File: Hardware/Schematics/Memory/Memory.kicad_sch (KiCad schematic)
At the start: 5 parts

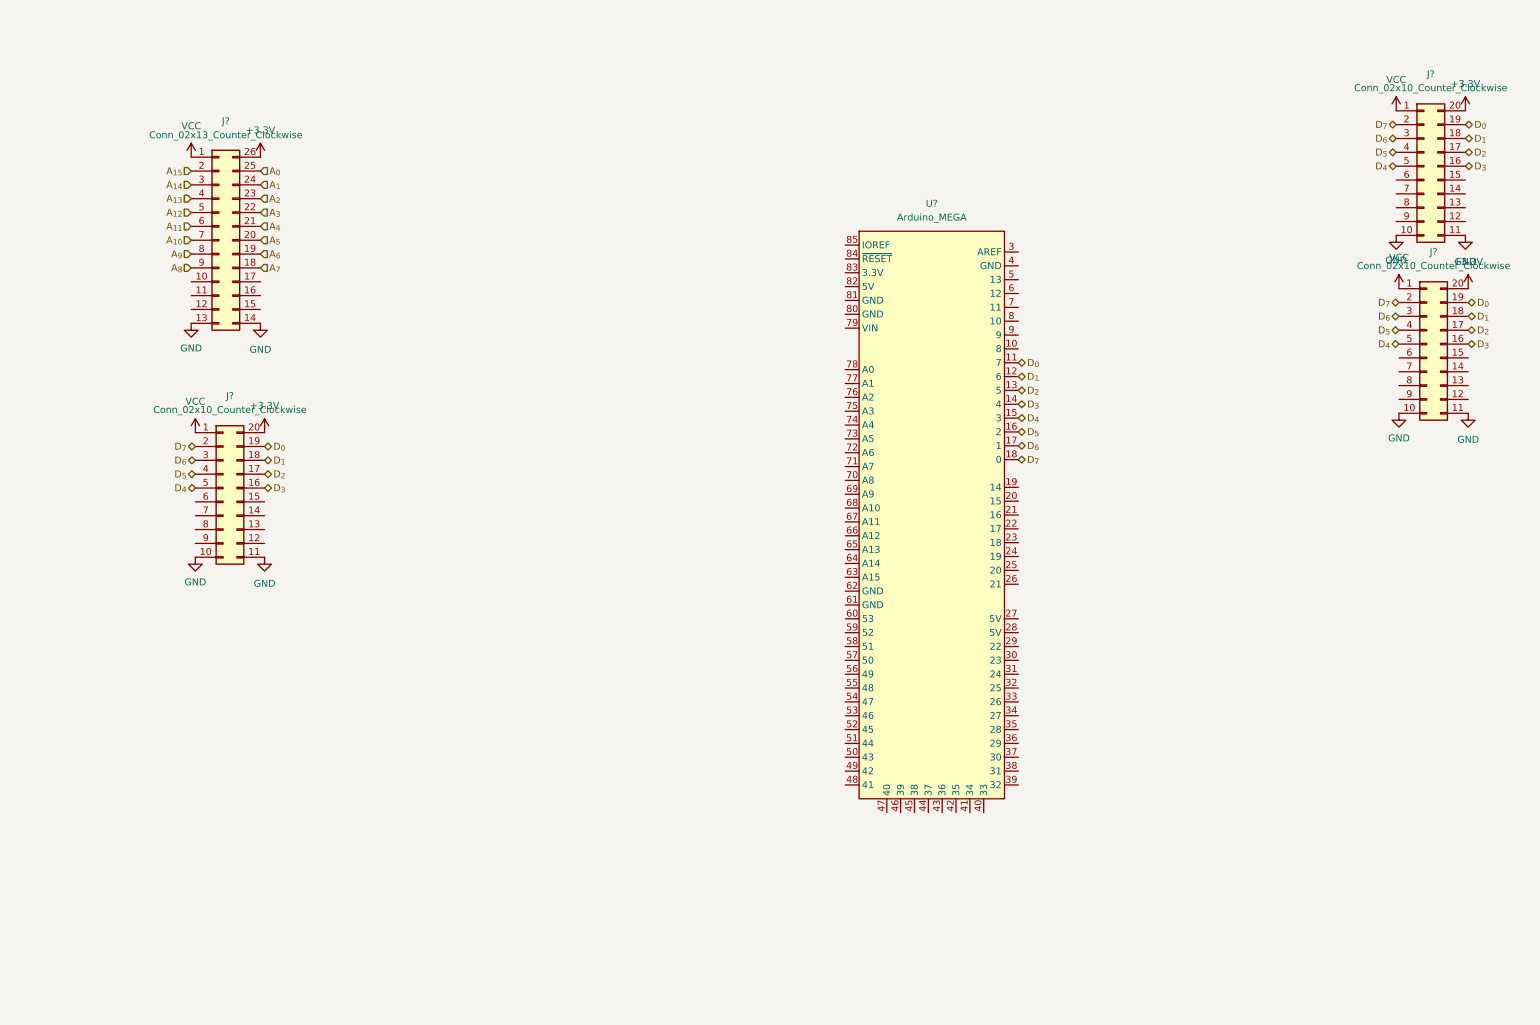
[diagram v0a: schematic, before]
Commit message: Updated Schematics
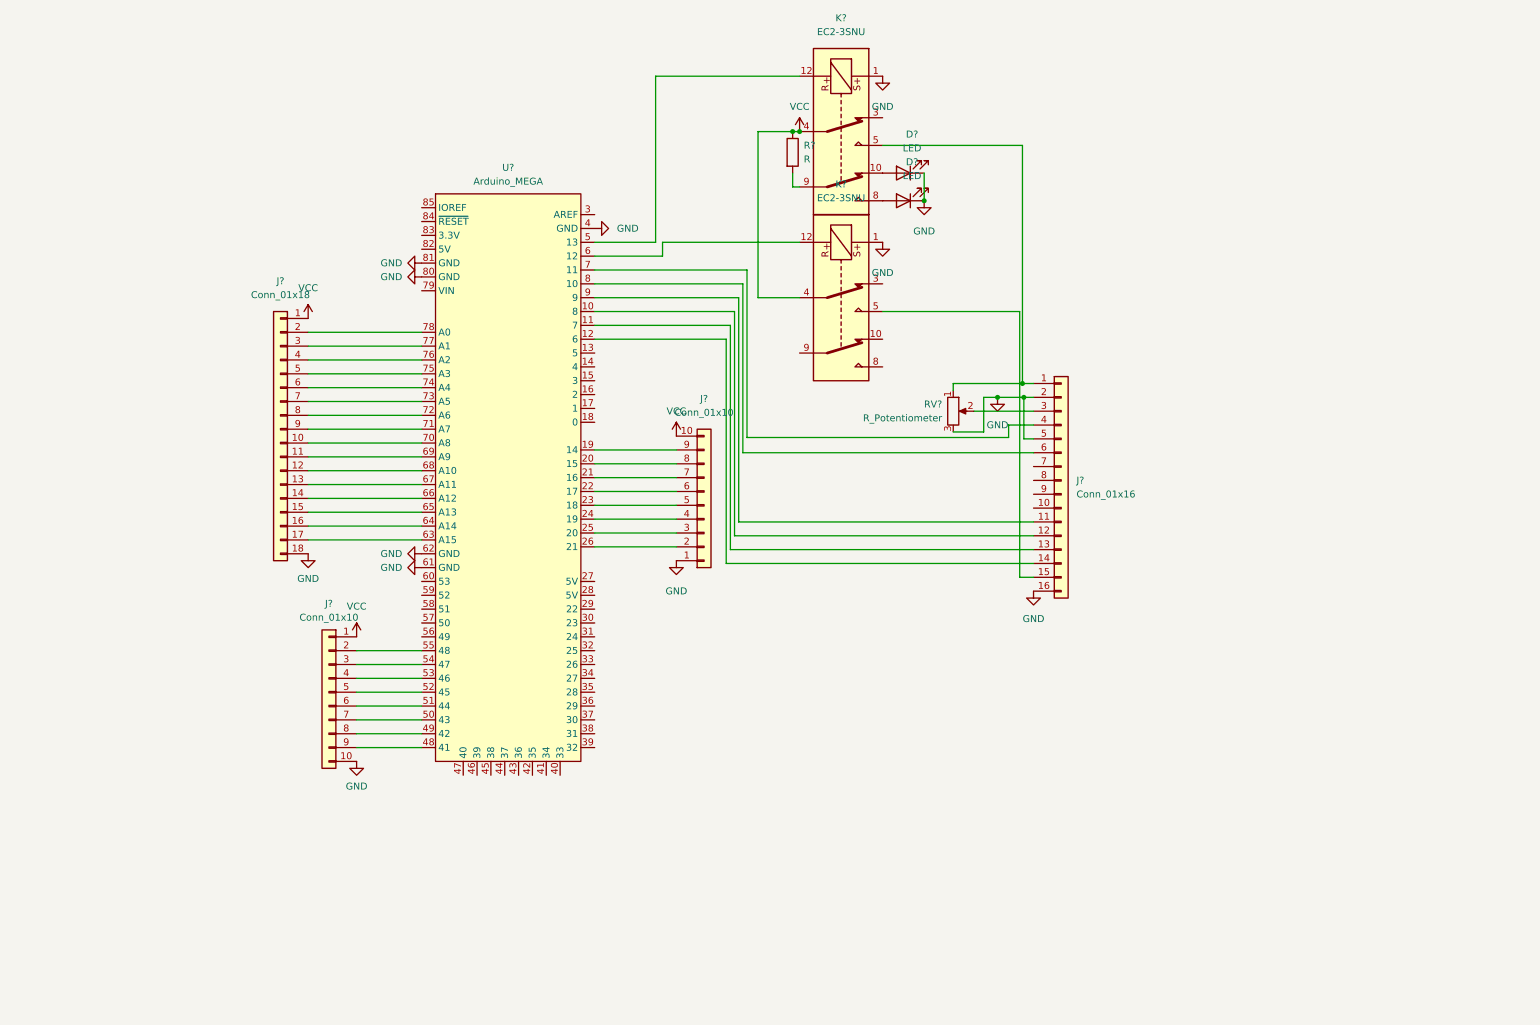
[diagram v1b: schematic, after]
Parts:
- removed J? (x3): Conn_02x10_Counter_Clockwise, Connector_PinSocket_2.54mm:PinSocket_2x10_P2.54mm_Horizontal, symbol Connector_Generic:Conn_02x10_Counter_Clockwise
- removed J?: Conn_02x13_Counter_Clockwise, Connector_PinHeader_2.54mm:PinHeader_2x13_P2.54mm_Horizontal, symbol Connector_Generic:Conn_02x13_Counter_Clockwise
- removed U?: Arduino_MEGA, symbol MyCustomLib:Arduino_MEGA
- added D? (x2): LED, symbol Device:LED
- added J? (x2): Conn_01x10, symbol Connector_Generic:Conn_01x10
- added J?: Conn_01x16, symbol Connector_Generic:Conn_01x16
- added J?: Conn_01x18, symbol Connector_Generic:Conn_01x18
- added K? (x2): EC2-3SNU, Relay_THT:Relay_DPDT_Kemet_EC2, symbol Relay:EC2-3SNU
- added R?: R, symbol Device:R
- added RV?: R_Potentiometer, symbol Device:R_Potentiometer
- added U?: Arduino_MEGA, symbol MyCustomLib:Arduino_MEGA
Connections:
- net GND: now also D?.1 (K), D?.1 (K), J?.1 (Pin_1), J?.10 (Pin_10), J?.16 (Pin_16), J?.18 (Pin_18), J?.2 (Pin_2), J?.5 (Pin_5), K?.1, K?.1, RV?.3, U?.4 (GND), U?.61 (GND), U?.62 (GND), U?.80 (GND), U?.81 (GND)
- net VCC: now also J?.1 (Pin_1), J?.1 (Pin_1), J?.10 (Pin_10), K?.4, K?.4, R?.1
- new net: D?.2 (A), K?.10
- new net: K?.12, U?.5 (13)
- new net: J?.1 (Pin_1), K?.5, RV?.1
- new net: D?.2 (A), K?.8
- new net: K?.9, R?.2
- new net: J?.2 (Pin_2), U?.55 (48)
- new net: J?.3 (Pin_3), U?.54 (47)
- new net: J?.4 (Pin_4), U?.53 (46)
- new net: J?.5 (Pin_5), U?.52 (45)
- new net: J?.6 (Pin_6), U?.51 (44)
- new net: J?.7 (Pin_7), U?.50 (43)
- new net: J?.8 (Pin_8), U?.49 (42)
- new net: J?.9 (Pin_9), U?.48 (41)
- new net: K?.12, U?.6 (12)
- new net: J?.15 (Pin_15), K?.5
- new net: J?.11 (Pin_11), U?.9
- new net: J?.12 (Pin_12), U?.10 (8)
- new net: J?.13 (Pin_13), U?.11 (7)
- new net: J?.14 (Pin_14), U?.12 (6)
- new net: J?.3 (Pin_3), RV?.2
- new net: J?.4 (Pin_4), U?.7 (11)
- new net: J?.6 (Pin_6), U?.8 (10)
- new net: J?.10 (Pin_10), U?.70 (A8)
- new net: J?.11 (Pin_11), U?.69 (A9)
- new net: J?.12 (Pin_12), U?.68 (A10)
- new net: J?.13 (Pin_13), U?.67 (A11)
- new net: J?.14 (Pin_14), U?.66 (A12)
- new net: J?.15 (Pin_15), U?.65 (A13)
- new net: J?.16 (Pin_16), U?.64 (A14)
- new net: J?.17 (Pin_17), U?.63 (A15)
- new net: J?.2 (Pin_2), U?.78 (A0)
- new net: J?.3 (Pin_3), U?.77 (A1)
- new net: J?.4 (Pin_4), U?.76 (A2)
- new net: J?.5 (Pin_5), U?.75 (A3)
- new net: J?.6 (Pin_6), U?.74 (A4)
- new net: J?.7 (Pin_7), U?.73 (A5)
- new net: J?.8 (Pin_8), U?.72 (A6)
- new net: J?.9 (Pin_9), U?.71 (A7)
- new net: J?.9 (Pin_9), U?.19 (14)
- new net: J?.8 (Pin_8), U?.20 (15)
- new net: J?.7 (Pin_7), U?.21 (16)
- new net: J?.6 (Pin_6), U?.22 (17)
- new net: J?.5 (Pin_5), U?.23 (18)
- new net: J?.4 (Pin_4), U?.24 (19)
- new net: J?.3 (Pin_3), U?.25 (20)
- new net: J?.2 (Pin_2), U?.26 (21)

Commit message: Updated All Schematics to be up-to-date
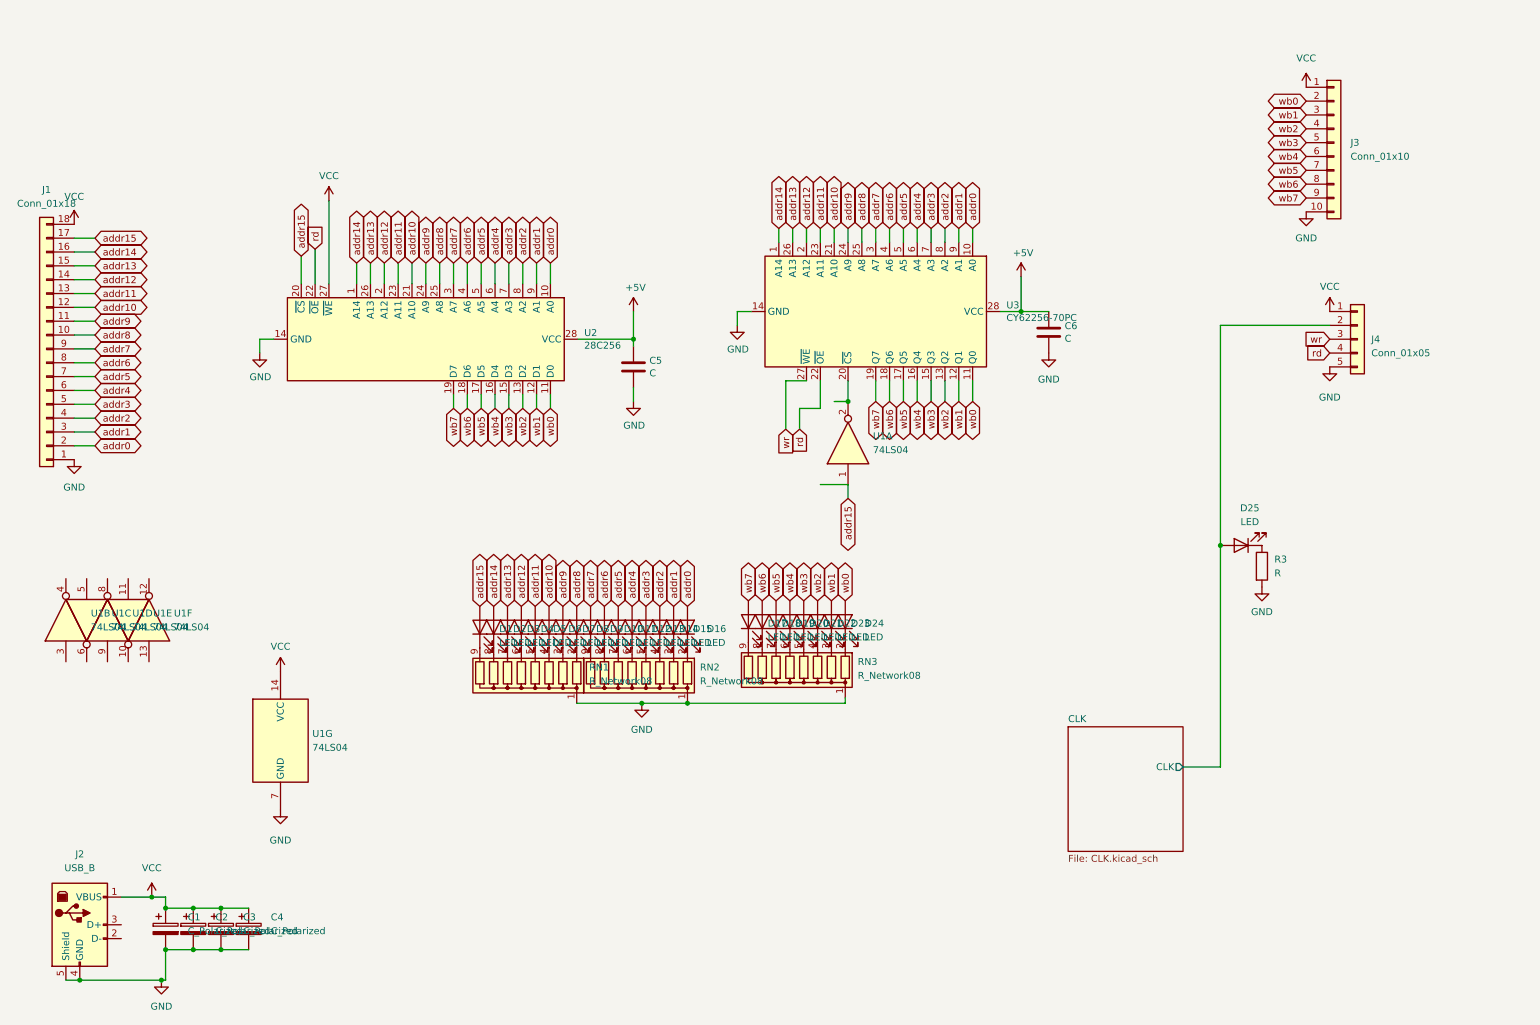
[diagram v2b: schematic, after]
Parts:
- removed D? (x2): LED, symbol Device:LED
- removed J? (x2): Conn_01x10, symbol Connector_Generic:Conn_01x10
- removed J?: Conn_01x16, symbol Connector_Generic:Conn_01x16
- removed J?: Conn_01x18, symbol Connector_Generic:Conn_01x18
- removed K? (x2): EC2-3SNU, Relay_THT:Relay_DPDT_Kemet_EC2, symbol Relay:EC2-3SNU
- removed R?: R, symbol Device:R
- removed RV?: R_Potentiometer, symbol Device:R_Potentiometer
- removed U?: Arduino_MEGA, symbol MyCustomLib:Arduino_MEGA
- added C1, C2, C3, C4: C_Polarized, Capacitor_THT:CP_Radial_D8.0mm_P3.80mm, symbol Device:C_Polarized
- added C5, C6: C, Capacitor_THT:C_Disc_D3.0mm_W2.0mm_P2.50mm, symbol Device:C
- added D1, D10, D11, D12, D13, D14, D15, D16, D17, D18, D19, D2, D20, D21, D22, D23, D24, D25, D3, D4, D5, D6, D7, D8, D9: LED, LED_THT:LED_D3.0mm, symbol Device:LED
- added J1: Conn_01x18, Connector_PinHeader_2.54mm:PinHeader_1x18_P2.54mm_Vertical, symbol Connector_Generic:Conn_01x18
- added J2: USB_B, Connector_USB:USB_B_Lumberg_2411_02_Horizontal, symbol Connector:USB_B
- added J3: Conn_01x10, Connector_PinHeader_2.54mm:PinHeader_1x10_P2.54mm_Vertical, symbol Connector_Generic:Conn_01x10
- added J4: Conn_01x05, Connector_PinHeader_2.54mm:PinHeader_1x05_P2.54mm_Vertical, symbol Connector_Generic:Conn_01x05
- added R3: R, Resistor_THT:R_Axial_DIN0204_L3.6mm_D1.6mm_P2.54mm_Vertical, symbol Device:R
- added RN1, RN2, RN3: R_Network08, Resistor_THT:R_Array_SIP9, symbol Device:R_Network08
- added U1: 74LS04, Package_DIP:DIP-14_W7.62mm_Socket_LongPads, symbol 74xx:74LS04
- added U2: 28C256, Package_DIP:DIP-28_W15.24mm, symbol Memory_EEPROM:28C256
- added U3: CY62256-70PC, Package_DIP:DIP-28_W15.24mm, symbol Memory_RAM:CY62256-70PC
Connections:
- net GND: now also C1.2, C2.2, C3.2, C4.2, C5.2, C6.2, J1.1 (Pin_1), J2.4 (GND), J2.5 (Shield), J3.10 (Pin_10), J4.5 (Pin_5), R3.2, RN1.1 (common), RN2.1 (common), RN3.1 (common), U1.7 (GND), U2.14 (GND), U3.14 (GND)
- net VCC: now also C1.1, C2.1, C3.1, C4.1, J1.18 (Pin_18), J2.1 (VBUS), J3.1 (Pin_1), J4.1 (Pin_1), U1.14 (VCC), U2.27 (~{WE})
- new net: D22.1 (K), RN3.4 (R3)
- new net: D24.1 (K), RN3.2 (R1)
- new net: D23.1 (K), RN3.3 (R2)
- new net: D21.1 (K), RN3.5 (R4)
- new net: D20.1 (K), RN3.6 (R5)
- new net: D19.1 (K), RN3.7 (R6)
- new net: D18.1 (K), RN3.8 (R7)
- new net: D17.1 (K), RN3.9 (R8)
- new net: D15.1 (K), RN2.3 (R2)
- new net: D3.1 (K), RN1.7 (R6)
- new net: D10.1 (K), RN2.8 (R7)
- new net: D8.1 (K), RN1.2 (R1)
- new net: D7.1 (K), RN1.3 (R2)
- new net: D6.1 (K), RN1.4 (R3)
- new net: D5.1 (K), RN1.5 (R4)
- new net: D4.1 (K), RN1.6 (R5)
- new net: D2.1 (K), RN1.8 (R7)
- new net: D1.1 (K), RN1.9 (R8)
- new net: D14.1 (K), RN2.4 (R3)
- new net: D25.1 (K), R3.1
- new net: D16.1 (K), RN2.2 (R1)
- new net: D13.1 (K), RN2.5 (R4)
- new net: D12.1 (K), RN2.6 (R5)
- new net: D11.1 (K), RN2.7 (R6)
- new net: D9.1 (K), RN2.9 (R8)
- new net: U1.2, U3.20 (~{CS})
- new net +5V: C5.1, C6.1, U2.28 (VCC), U3.28 (VCC)
- new net CLK/CLK: D25.2 (A), J4.2 (Pin_2)
- new net addr0: D16.2 (A), J1.2 (Pin_2), U2.10 (A0), U3.10 (A0)
- new net addr1: D15.2 (A), J1.3 (Pin_3), U2.9 (A1), U3.9 (A1)
- new net addr10: D6.2 (A), J1.12 (Pin_12), U2.21 (A10), U3.21 (A10)
- new net addr11: D5.2 (A), J1.13 (Pin_13), U2.23 (A11), U3.23 (A11)
- new net addr12: D4.2 (A), J1.14 (Pin_14), U2.2 (A12), U3.2 (A12)
- new net addr13: D3.2 (A), J1.15 (Pin_15), U2.26 (A13), U3.26 (A13)
- new net addr14: D2.2 (A), J1.16 (Pin_16), U2.1 (A14), U3.1 (A14)
- new net addr15: D1.2 (A), J1.17 (Pin_17), U1.1, U2.20 (~{CS})
- new net addr2: D14.2 (A), J1.4 (Pin_4), U2.8 (A2), U3.8 (A2)
- new net addr3: D13.2 (A), J1.5 (Pin_5), U2.7 (A3), U3.7 (A3)
- new net addr4: D12.2 (A), J1.6 (Pin_6), U2.6 (A4), U3.6 (A4)
- new net addr5: D11.2 (A), J1.7 (Pin_7), U2.5 (A5), U3.5 (A5)
- new net addr6: D10.2 (A), J1.8 (Pin_8), U2.4 (A6), U3.4 (A6)
- new net addr7: D9.2 (A), J1.9 (Pin_9), U2.3 (A7), U3.3 (A7)
- new net addr8: D8.2 (A), J1.10 (Pin_10), U2.25 (A8), U3.25 (A8)
- new net addr9: D7.2 (A), J1.11 (Pin_11), U2.24 (A9), U3.24 (A9)
- new net rd: J4.4 (Pin_4), U2.22 (~{OE}), U3.22 (~{OE})
- new net wb0: D24.2 (A), J3.2 (Pin_2), U2.11 (D0), U3.11 (Q0)
- new net wb1: D23.2 (A), J3.3 (Pin_3), U2.12 (D1), U3.12 (Q1)
- new net wb2: D22.2 (A), J3.4 (Pin_4), U2.13 (D2), U3.13 (Q2)
- new net wb3: D21.2 (A), J3.5 (Pin_5), U2.15 (D3), U3.15 (Q3)
- new net wb4: D20.2 (A), J3.6 (Pin_6), U2.16 (D4), U3.16 (Q4)
- new net wb5: D19.2 (A), J3.7 (Pin_7), U2.17 (D5), U3.17 (Q5)
- new net wb6: D18.2 (A), J3.8 (Pin_8), U2.18 (D6), U3.18 (Q6)
- new net wb7: D17.2 (A), J3.9 (Pin_9), U2.19 (D7), U3.19 (Q7)
- new net wr: J4.3 (Pin_3), U3.27 (~{WE})
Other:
- added sheet CLK (CLK.kicad_sch)
